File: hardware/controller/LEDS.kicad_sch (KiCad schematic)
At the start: 22 parts, among them IC2 PCA9685PW_Q900,118

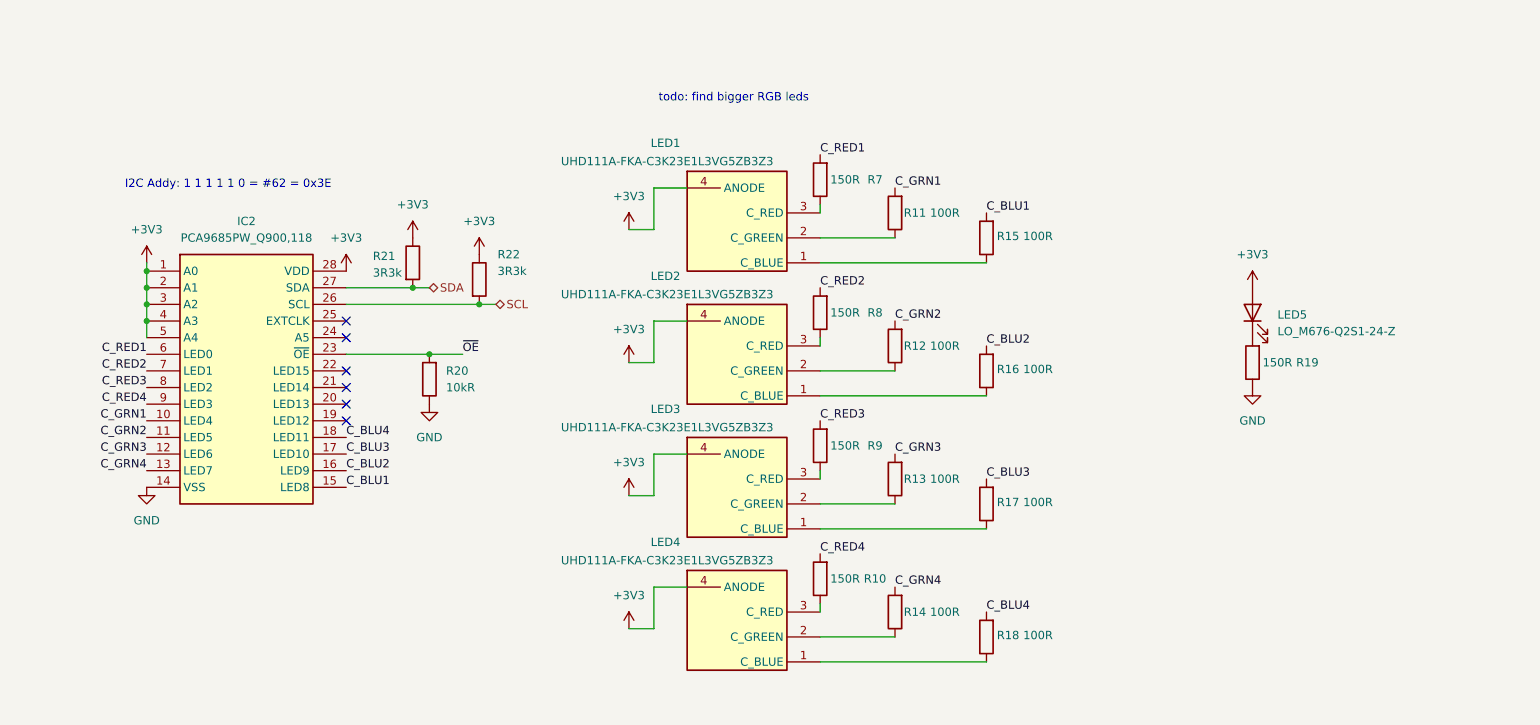
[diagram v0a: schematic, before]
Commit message: fixed bus stuff
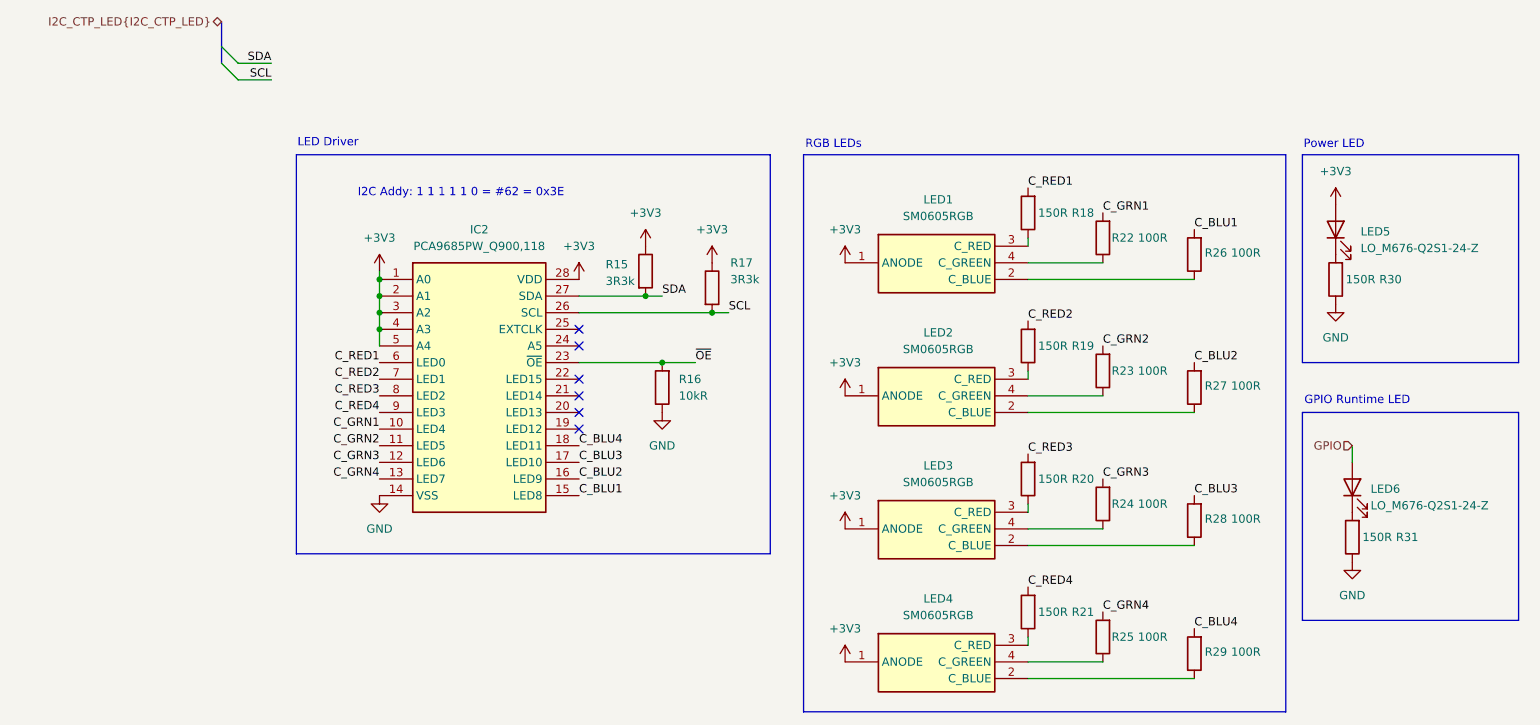
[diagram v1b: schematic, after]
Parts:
- removed LED1, LED2, LED3, LED4: UHD111A-FKA-C3K23E1L3VG5ZB3Z3, UHD111AFKAC3K23E1L3VG5ZB3Z3, symbol SamacSys_Parts:UHD111A-FKA-C3K23E1L3VG5ZB3Z3
- added LED1, LED2, LED3, LED4: SM0605RGB, SM0605RGB, symbol SamacSys_Parts:SM0605RGB
- added LED6: LO_M676-Q2S1-24-Z, LEDM2214X140N, symbol Device:LED
- added R31: 150R, RESC2012X60N, symbol Device:R
- renumbered R21 to R15, R20 to R16, R22 to R17, R7 to R18, R8 to R19, R9 to R20, R10 to R21, R11 to R22, R12 to R23, R13 to R24, R14 to R25, R15 to R26, R16 to R27, R17 to R28, R18 to R29, R19 to R30
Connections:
- net +3V3: now also LED1.1 (ANODE), LED2.1 (ANODE), LED3.1 (ANODE), LED4.1 (ANODE)
- net GND: now also R31.1
- net at R25.1: now also LED4.4 (C_GREEN)
- net at R26.1: now also LED1.2 (C_BLUE)
- net at R22.1: now also LED1.4 (C_GREEN)
- net at R18.1: now also LED1.3 (C_RED)
- net at R29.1: now also LED4.2 (C_BLUE)
- net at R21.1: now also LED4.3 (C_RED)
- net at R28.1: now also LED3.2 (C_BLUE)
- net at R19.1: now also LED2.3 (C_RED)
- net at R24.1: now also LED3.4 (C_GREEN)
- net at R20.1: now also LED3.3 (C_RED)
- net at R27.1: now also LED2.2 (C_BLUE)
- net at R23.1: now also LED2.4 (C_GREEN)
- new net: LED6.1 (K), R31.2
- new net GPIO: LED6.2 (A)
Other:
- note added: "GPIO Runtime LED"
- note added: "LED Driver"
- note added: "Power LED"
- note added: "RGB LEDs"
- note removed: "todo: find bigger RGB leds"
- moved on the sheet: IC2, LED5, R15, R16, R17, R18, R19, R20, R21, R22, R23, R24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
